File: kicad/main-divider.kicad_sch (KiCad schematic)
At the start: 27 parts, among them U11 TL074, U12 CD4024

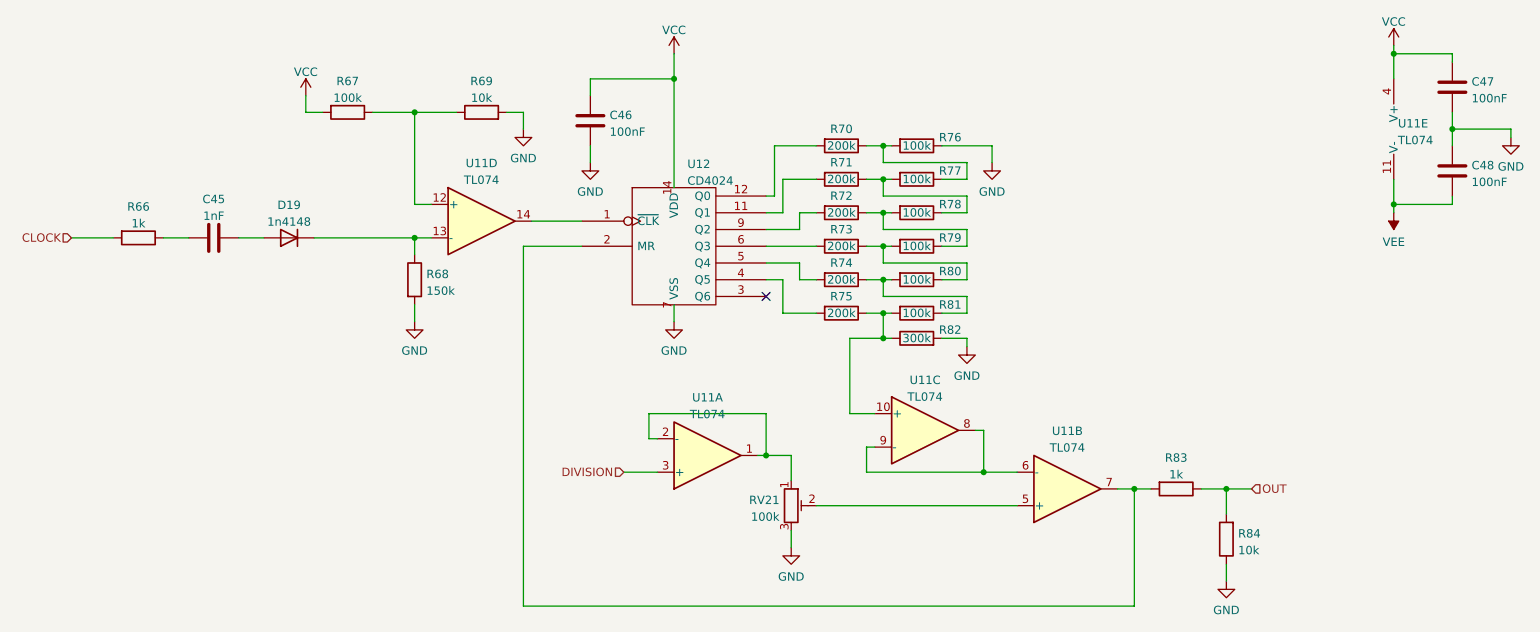
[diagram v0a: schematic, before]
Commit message: Final changes for rev01
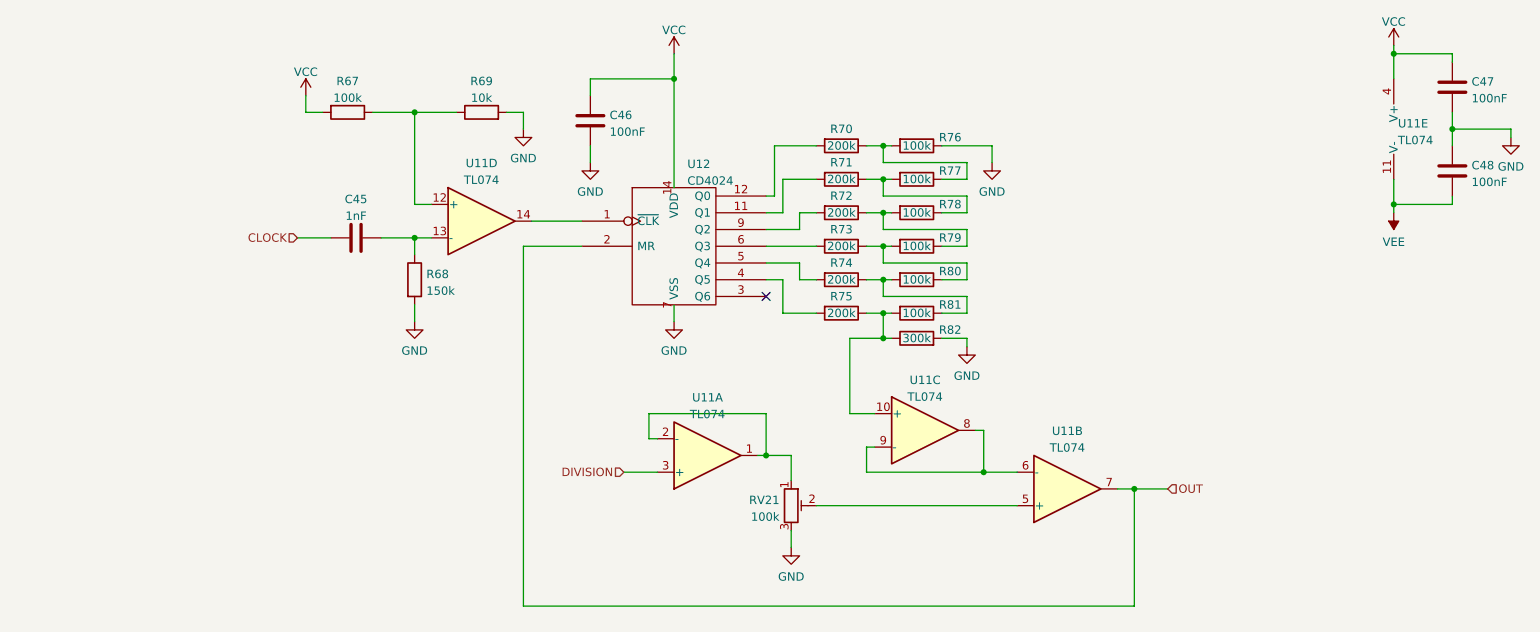
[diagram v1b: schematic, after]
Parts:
- removed D19: 1n4148, rumblesan-standard-parts:D_DO-35_SOD27_P7.62mm_Horizontal, symbol Device:D
- removed R66, R83: 1k, rumblesan-standard-parts:R_Axial_DIN0207_L6.3mm_D2.5mm_P10.16mm_Horizontal, symbol rumblesan-standard-parts:R
- removed R84: 10k, rumblesan-standard-parts:R_Axial_DIN0207_L6.3mm_D2.5mm_P10.16mm_Horizontal, symbol rumblesan-standard-parts:R
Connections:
- net CLOCK: now also C45.1
- net OUT: now also U11.7, U12.2 (MR)
- net at C45.2: now also R68.1, U11.13 (-)
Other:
- moved on the sheet: C45
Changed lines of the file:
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@@
   (junction (at 233.68 63.5) (diameter 0) (color 0 0 0 0)
-  )
-  (junction (at 208.28 106.68) (diameter 0) (color 0 0 0 0)
   )
   (junction (at 194.31 106.68) (diameter 0) (color 0 0 0 0)
@@
     (stroke (width 0) (type default) (color 0 0 0 0))
   )
-  (wire (pts (xy 208.28 118.11) (xy 208.28 120.65))
-    (stroke (width 0) (type default) (color 0 0 0 0))
-  )
   (wire (pts (xy 85.09 49.53) (xy 91.44 49.53))
     (stroke (width 0) (type default) (color 0 0 0 0))
@@
     (stroke (width 0) (type default) (color 0 0 0 0))
   )
-  (wire (pts (xy 33.02 68.58) (xy 39.37 68.58))
-    (stroke (width 0) (type default) (color 0 0 0 0))
-  )
   (wire (pts (xy 137.16 101.6) (xy 138.43 101.6))
     (stroke (width 0) (type default) (color 0 0 0 0))
   )
-  (wire (pts (xy 194.31 106.68) (xy 196.85 106.68))
+  (wire (pts (xy 194.31 106.68) (xy 199.39 106.68))
     (stroke (width 0) (type default) (color 0 0 0 0))
   )
@@
     (stroke (width 0) (type default) (color 0 0 0 0))
   )
-  (wire (pts (xy 208.28 106.68) (xy 212.09 106.68))
-    (stroke (width 0) (type default) (color 0 0 0 0))
-  )
   (wire (pts (xy 165.1 59.69) (xy 168.91 59.69))
     (stroke (width 0) (type default) (color 0 0 0 0))
   )
-  (wire (pts (xy 58.42 68.58) (xy 62.23 68.58))
+  (wire (pts (xy 80.01 68.58) (xy 85.09 68.58))
     (stroke (width 0) (type default) (color 0 0 0 0))
   )
@@
     (stroke (width 0) (type default) (color 0 0 0 0))
   )
-  (wire (pts (xy 204.47 106.68) (xy 208.28 106.68))
-    (stroke (width 0) (type default) (color 0 0 0 0))
-  )
   (wire (pts (xy 85.09 49.53) (xy 85.09 63.5))
     (stroke (width 0) (type default) (color 0 0 0 0))
   )
-  (wire (pts (xy 69.85 68.58) (xy 85.09 68.58))
-    (stroke (width 0) (type default) (color 0 0 0 0))
-  )
   (wire (pts (xy 156.21 83.82) (xy 157.48 83.82))
     (stroke (width 0) (type default) (color 0 0 0 0))
@@
     (stroke (width 0) (type default) (color 0 0 0 0))
   )
-  (wire (pts (xy 46.99 68.58) (xy 50.8 68.58))
+  (wire (pts (xy 67.31 68.58) (xy 72.39 68.58))
     (stroke (width 0) (type default) (color 0 0 0 0))
   )
@@
   )
   (wire (pts (xy 101.6 69.85) (xy 101.6 124.46))
-    (stroke (width 0) (type default) (color 0 0 0 0))
-  )
-  (wire (pts (xy 208.28 106.68) (xy 208.28 110.49))
     (stroke (width 0) (type default) (color 0 0 0 0))
   )
@@
     (effects (font (size 1.27 1.27)) (justify right))
   )
-  (hierarchical_label "CLOCK" (shape input) (at 33.02 68.58 180)
+  (hierarchical_label "CLOCK" (shape input) (at 67.31 68.58 180)
     (effects (font (size 1.27 1.27)) (justify right))
   )
-  (hierarchical_label "OUT" (shape input) (at 212.09 106.68 0)
+  (hierarchical_label "OUT" (shape input) (at 199.39 106.68 0)
     (effects (font (size 1.27 1.27)) (justify left))
   )
@@
     (pin "1")
   )
-  (symbol (lib_id "rumblesan-standard-parts:C") (at 54.61 68.58 90) (unit 1)
-    (in_bom yes) (on_board yes) (fields_autoplaced)
-    (property "Reference" "C45" (id 0) (at 54.61 62.7212 90))
-    (property "Value" "1nF" (id 1) (at 54.61 65.2581 90))
-    (property "Footprint" "rumblesan-standard-parts:C_Rect_L7.0mm_W2.5mm_P5.00mm" (id 2) (at 53.34 62.865 90)
-      (effects (font (size 1.27 1.27)) hide)
-    )
-    (property "Datasheet" "~" (id 3) (at 54.61 60.96 90)
-      (effects (font (size 1.27 1.27)) hide)
-    )
-    (property "Spec" "ceramic C0G" (id 4) (at 54.61 64.77 90)
-      (effects (font (size 1.27 1.27)) hide)
-    )
-    (property "Tolerance" "5%" (id 5) (at 46.355 64.77 90)
-      (effects (font (size 1.27 1.27)) hide)
-    )
-    (pin "1")
-    (pin "2")
-  )
-  (symbol (lib_id "rumblesan-standard-parts:R") (at 43.18 68.58 90) (unit 1)
-    (in_bom yes) (on_board yes) (fields_autoplaced)
-    (property "Reference" "R66" (id 0) (at 43.18 63.8642 90))
-    (property "Value" "1k" (id 1) (at 43.18 66.4011 90))
-    (property "Footprint" "rumblesan-standard-parts:R_Axial_DIN0207_L6.3mm_D2.5mm_P10.16mm_Horizontal" (id 2) (at 45.72 66.04 90)
-      (effects (font (size 1.27 1.27)) hide)
-    )
-    (property "Datasheet" "~" (id 3) (at 43.18 62.23 90)
-      (effects (font (size 1.27 1.27)) hide)
-    )
-    (property "Tolerance" "1%" (id 4) (at 49.53 63.5 90)
-      (effects (font (size 1.27 1.27)) hide)
-    )
-    (property "Power" "0.5W" (id 5) (at 35.56 63.5 90)
-      (effects (font (size 1.27 1.27)) hide)
-    )
-    (property "Spec" "metal film" (id 6) (at 43.18 63.5 90)
+  (symbol (lib_id "rumblesan-standard-parts:C") (at 76.2 68.58 90) (unit 1)
+    (in_bom yes) (on_board yes) (fields_autoplaced)
+    (property "Reference" "C45" (id 0) (at 76.2 62.7212 90))
+    (property "Value" "1nF" (id 1) (at 76.2 65.2581 90))
+    (property "Footprint" "rumblesan-standard-parts:C_Rect_L7.0mm_W2.5mm_P5.00mm" (id 2) (at 74.93 62.865 90)
+      (effects (font (size 1.27 1.27)) hide)
+    )
+    (property "Datasheet" "~" (id 3) (at 76.2 60.96 90)
+      (effects (font (size 1.27 1.27)) hide)
+    )
+    (property "Spec" "ceramic C0G" (id 4) (at 76.2 64.77 90)
+      (effects (font (size 1.27 1.27)) hide)
+    )
+    (property "Tolerance" "5%" (id 5) (at 67.945 64.77 90)
       (effects (font (size 1.27 1.27)) hide)
     )
@@
     (pin "2")
   )
-  (symbol (lib_id "rumblesan-standard-parts:R") (at 208.28 114.3 0) (unit 1)
-    (in_bom yes) (on_board yes) (fields_autoplaced)
-    (property "Reference" "R84" (id 0) (at 210.058 113.4653 0)
-      (effects (font (size 1.27 1.27)) (justify left))
-    )
-    (property "Value" "10k" (id 1) (at 210.058 116.0022 0)
-      (effects (font (size 1.27 1.27)) (justify left))
-    )
-    (property "Footprint" "rumblesan-standard-parts:R_Axial_DIN0207_L6.3mm_D2.5mm_P10.16mm_Horizontal" (id 2) (at 210.82 116.84 90)
-      (effects (font (size 1.27 1.27)) hide)
-    )
-    (property "Datasheet" "~" (id 3) (at 214.63 114.3 90)
-      (effects (font (size 1.27 1.27)) hide)
-    )
-    (property "Tolerance" "1%" (id 4) (at 213.36 120.65 90)
-      (effects (font (size 1.27 1.27)) hide)
-    )
-    (property "Power" "0.5W" (id 5) (at 213.36 106.68 90)
-      (effects (font (size 1.27 1.27)) hide)
-    )
-    (property "Spec" "metal film" (id 6) (at 213.36 114.3 90)
-      (effects (font (size 1.27 1.27)) hide)
-    )
-    (pin "1")
-    (pin "2")
-  )
   (symbol (lib_id "power:VCC") (at 124.46 40.64 0) (unit 1)
     (in_bom yes) (on_board yes) (fields_autoplaced)
@@
     )
     (property "Spec" "metal film" (id 6) (at 149.86 54.61 90)
-      (effects (font (size 1.27 1.27)) hide)
-    )
-    (pin "1")
-    (pin "2")
-  )
-  (symbol (lib_id "Device:D") (at 66.04 68.58 180) (unit 1)
-    (in_bom yes) (on_board yes) (fields_autoplaced)
-    (property "Reference" "D19" (id 0) (at 66.04 63.6102 0))
-    (property "Value" "1n4148" (id 1) (at 66.04 66.1471 0))
-    (property "Footprint" "rumblesan-standard-parts:D_DO-35_SOD27_P7.62mm_Horizontal" (id 2) (at 66.04 68.58 0)
-      (effects (font (size 1.27 1.27)) hide)
-    )
-    (property "Datasheet" "~" (id 3) (at 66.04 68.58 0)
       (effects (font (size 1.27 1.27)) hide)
     )
@@
     (pin "2")
   )
-  (symbol (lib_id "power:GND") (at 208.28 120.65 0) (unit 1)
-    (in_bom yes) (on_board yes) (fields_autoplaced)
-    (property "Reference" "#PWR0116" (id 0) (at 208.28 127 0)
-      (effects (font (size 1.27 1.27)) hide)
-    )
-    (property "Value" "GND" (id 1) (at 208.28 125.0934 0))
-    (property "Footprint" "" (id 2) (at 208.28 120.65 0)
-      (effects (font (size 1.27 1.27)) hide)
-    )
-    (property "Datasheet" "" (id 3) (at 208.28 120.65 0)
-      (effects (font (size 1.27 1.27)) hide)
-    )
-    (pin "1")
-  )
   (symbol (lib_id "rumblesan-standard-parts:R") (at 161.29 83.82 270) (unit 1)
     (in_bom yes) (on_board yes)
@@
       (effects (font (size 1.27 1.27)) hide)
     )
-    (pin "1")
-    (pin "2")
-  )
-  (symbol (lib_id "rumblesan-standard-parts:R") (at 200.66 106.68 90) (unit 1)
-    (in_bom yes) (on_board yes) (fields_autoplaced)
-    (property "Reference" "R83" (id 0) (at 200.66 101.9642 90))
-    (property "Value" "1k" (id 1) (at 200.66 104.5011 90))
-    (property "Footprint" "rumblesan-standard-parts:R_Axial_DIN0207_L6.3mm_D2.5mm_P10.16mm_Horizontal" (id 2) (at 203.2 104.14 90)
-      (effects (font (size 1.27 1.27)) hide)
-    )
-    (property "Datasheet" "~" (id 3) (at 200.66 100.33 90)
-      (effects (font (size 1.27 1.27)) hide)
-    )
-    (property "Tolerance" "1%" (id 4) (at 207.01 101.6 90)
-      (effects (font (size 1.27 1.27)) hide)
-    )
-    (property "Power" "0.5W" (id 5) (at 193.04 101.6 90)
-      (effects (font (size 1.27 1.27)) hide)
-    )
-    (property "Spec" "metal film" (id 6) (at 200.66 101.6 90)
-      (effects (font (size 1.27 1.27)) hide)
-    )
